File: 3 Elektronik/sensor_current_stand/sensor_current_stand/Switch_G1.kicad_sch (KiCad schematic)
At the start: 1 part, among them J5 DC37_Plug_MountingHoles

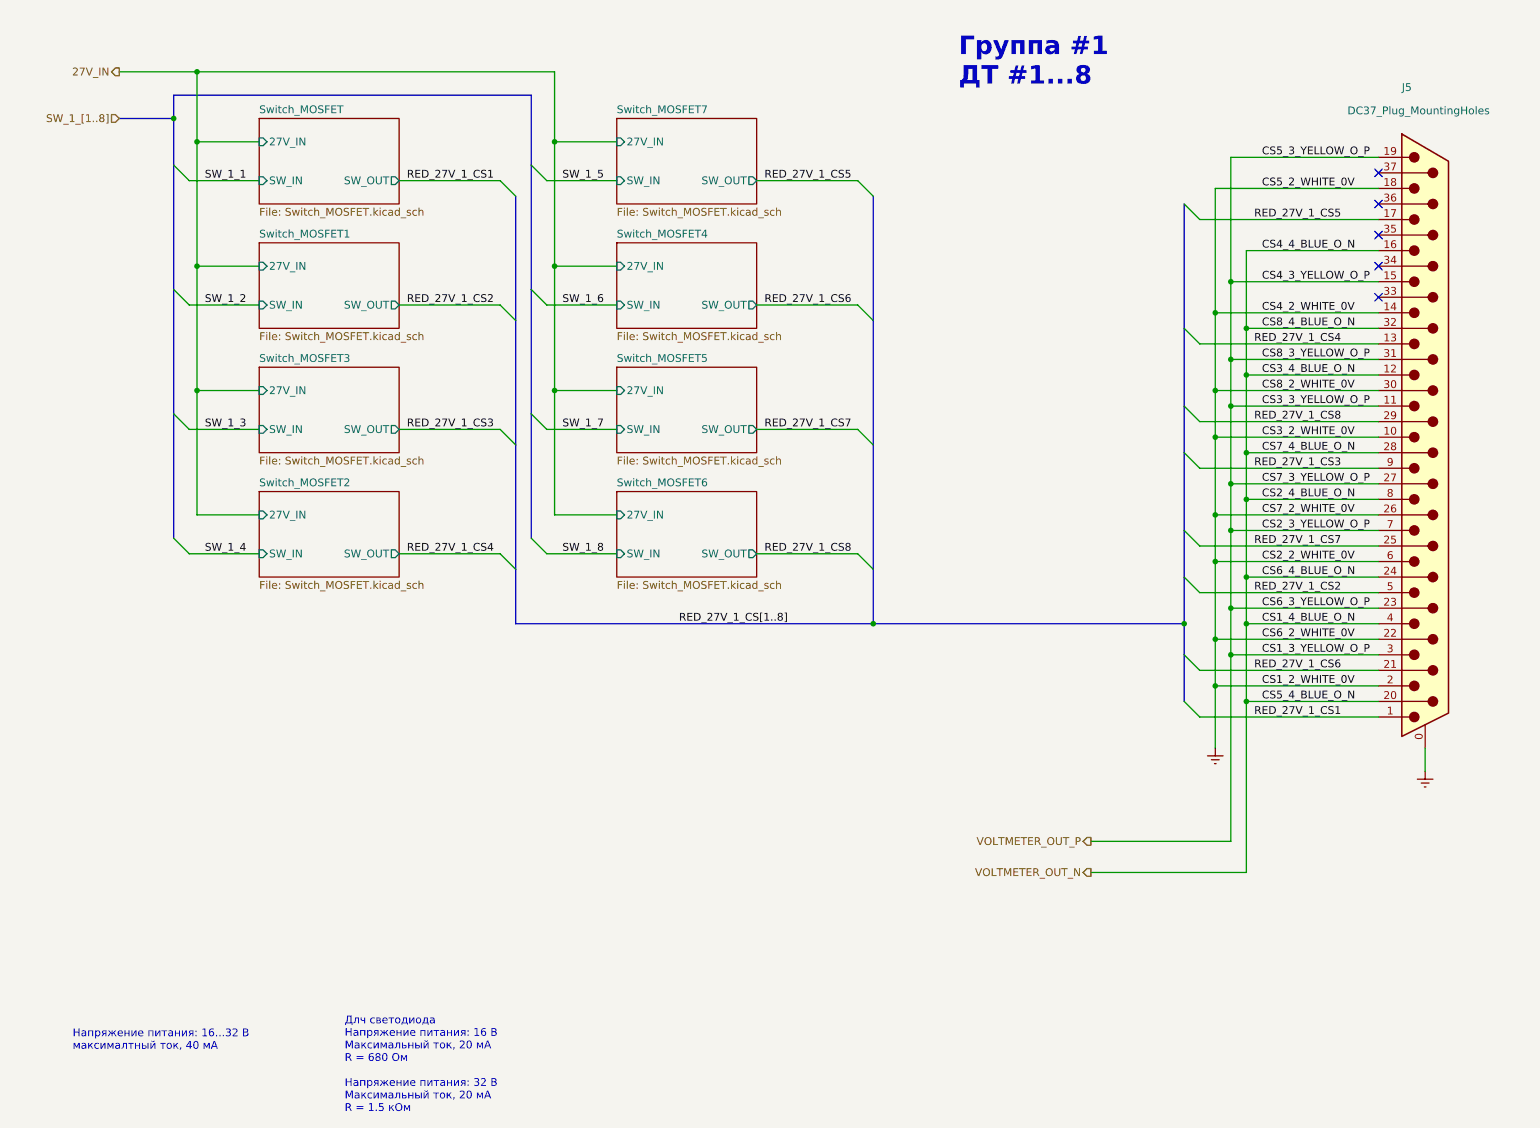
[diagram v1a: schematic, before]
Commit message: Version 2
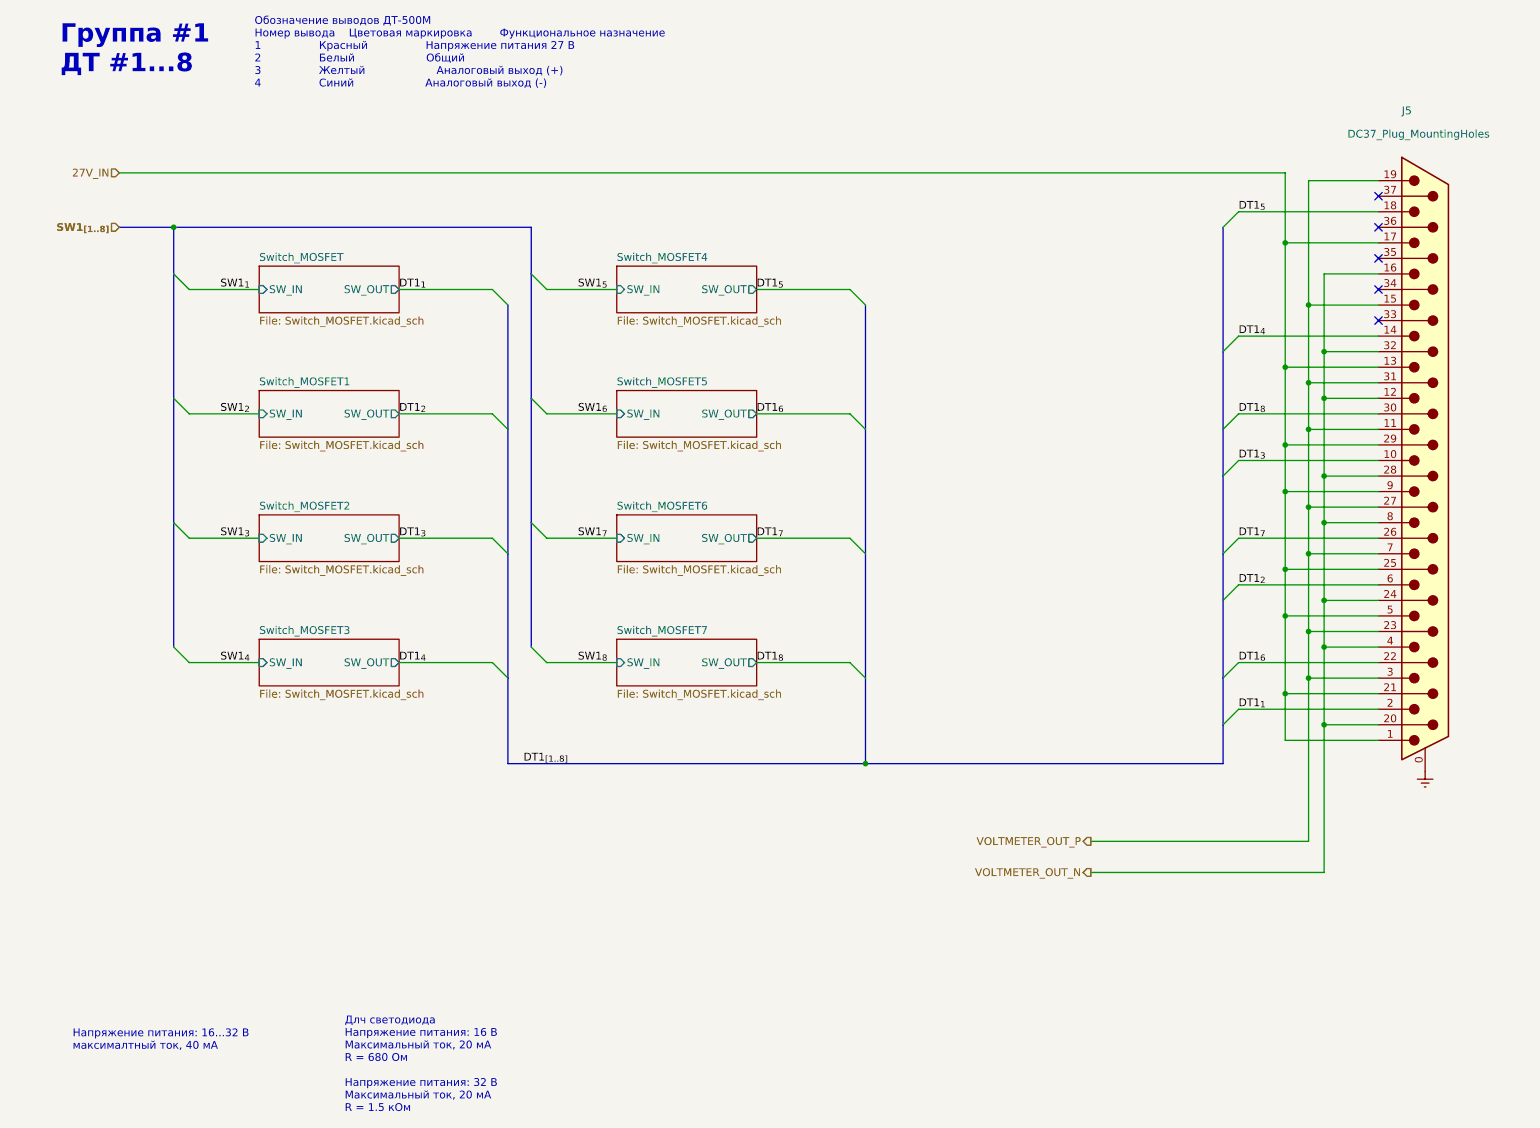
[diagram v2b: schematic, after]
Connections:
- net RED_27V_1_CS1 is gone; now on net 27V_IN: J5.1
- net RED_27V_1_CS2 is gone; now on net 27V_IN: J5.5
- net RED_27V_1_CS3 is gone; now on net 27V_IN: J5.9
- net RED_27V_1_CS4 is gone; now on net 27V_IN: J5.13
- net RED_27V_1_CS5 is gone; now on net 27V_IN: J5.17
- net RED_27V_1_CS6 is gone; now on net 27V_IN: J5.21
- net RED_27V_1_CS7 is gone; now on net 27V_IN: J5.25
- net RED_27V_1_CS8 is gone; now on net 27V_IN: J5.29
- net Earth: no longer J5.10, J5.14, J5.18, J5.2, J5.22, J5.26, J5.30, J5.6
- new net DT1_{1}: J5.2
- new net DT1_{2}: J5.6
- new net DT1_{3}: J5.10
- new net DT1_{4}: J5.14
- new net DT1_{5}: J5.18
- new net DT1_{6}: J5.22
- new net DT1_{7}: J5.26
- new net DT1_{8}: J5.30
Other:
- sheet Switch_MOSFET ports: added none; removed 27V_IN
- sheet Switch_MOSFET1 ports: added none; removed 27V_IN
- sheet Switch_MOSFET2 ports: added none; removed 27V_IN
- sheet Switch_MOSFET3 ports: added none; removed 27V_IN
- sheet Switch_MOSFET4 ports: added none; removed 27V_IN
- sheet Switch_MOSFET5 ports: added none; removed 27V_IN
- sheet Switch_MOSFET6 ports: added none; removed 27V_IN
- sheet Switch_MOSFET7 ports: added none; removed 27V_IN
- note added: "Обозначение выводов ДТ-500М Номер вывода Цветовая маркировка Функциональное назначение 1 Красный Напряжение питания 27 В 2 Белый Общий 3 Желтый Аналоговый выход (+) 4 Синий Аналоговый выход (-)"
- moved on the sheet: J5
